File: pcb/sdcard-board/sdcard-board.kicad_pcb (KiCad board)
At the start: 2 copper layers, 82.5 x 67.3 mm, 38 parts, among them J3 SD Card Board, J4 EXPBUS1, U1 74HC123, U3 74HC00, U4 74HC00, U5 74HC163, U6 74HC00, U7 74HC165, U8 74HC595, X1 16MHz

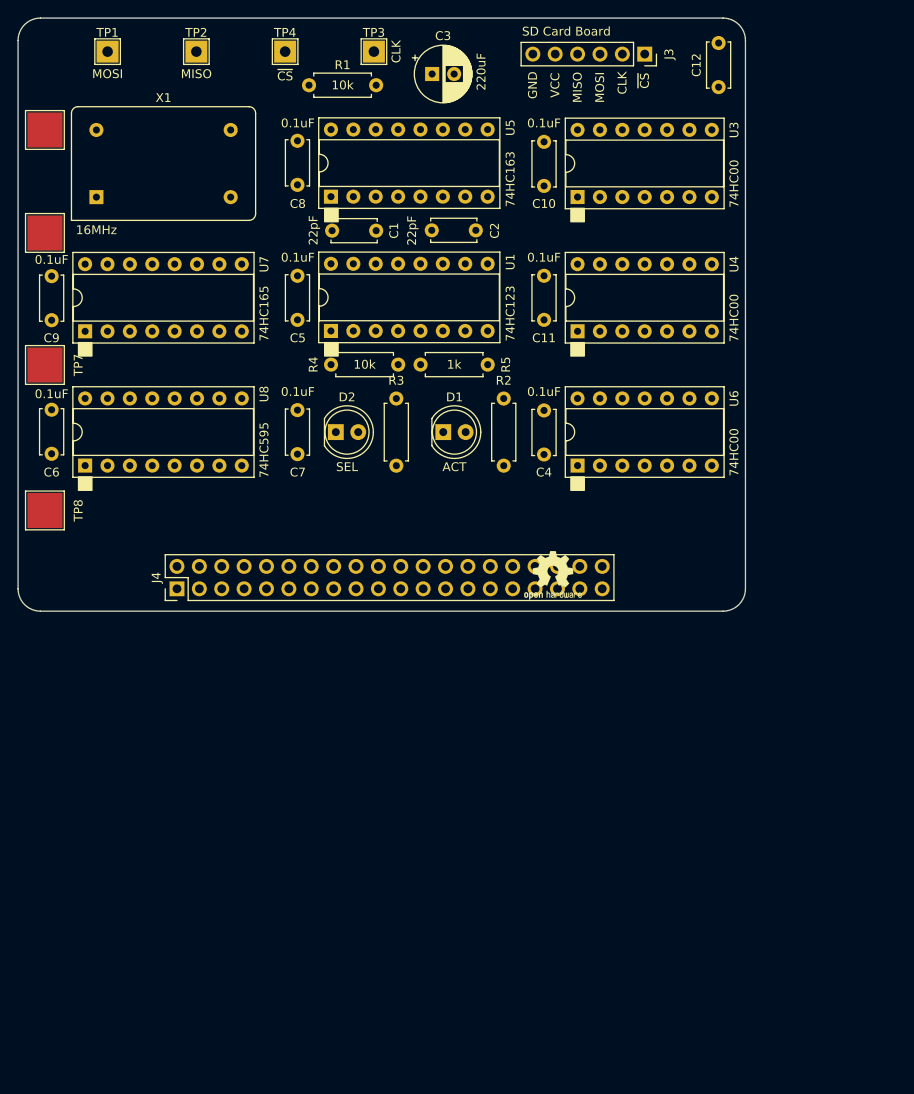
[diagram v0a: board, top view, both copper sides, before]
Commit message: Further redesigning boards
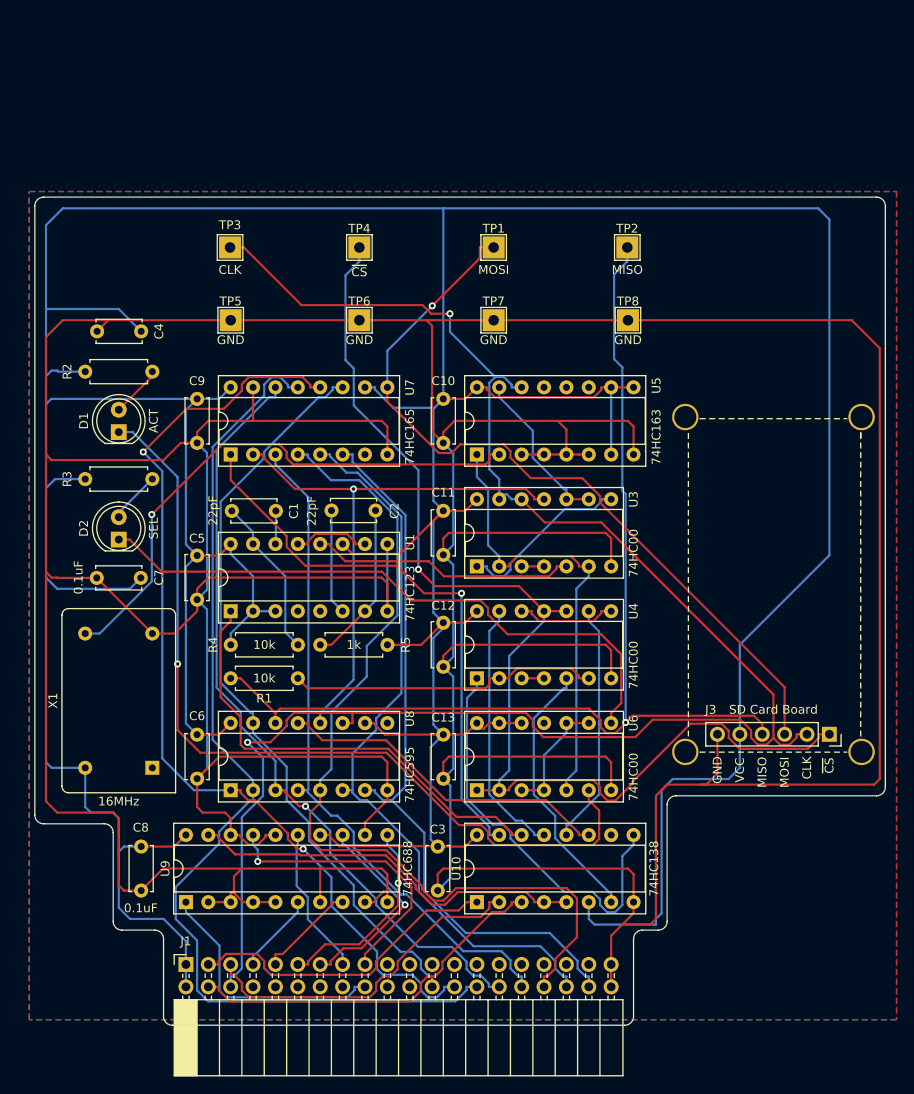
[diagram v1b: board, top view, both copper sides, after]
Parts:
- removed J4: EXPBUS1, Connector_PinHeader_2.54mm:PinHeader_2x20_P2.54mm_Vertical
- removed REF**: OSHW-Logo2_7.3x6mm_SilkScreen, Symbol:OSHW-Logo2_7.3x6mm_SilkScreen
- added C13: 0.1uF, Capacitor_THT:C_Disc_D5.0mm_W2.5mm_P5.00mm, F.Cu at (74.9, 115.6)
- added J1: EXPBUS2, Connector_PinSocket_2.54mm:PinSocket_2x20_P2.54mm_Horizontal, F.Cu at (45.7, 141.7)
- added U10: 74HC138, Package_DIP:DIP-16_W7.62mm_Socket, F.Cu at (78.7, 134.6)
- added U9: 74HC688, Package_DIP:DIP-20_W7.62mm_Socket, F.Cu at (45.7, 134.6)
- C3: value 220uF -> 0.1uF; footprint Capacitor_THT:CP_Radial_D6.3mm_P2.50mm -> Capacitor_THT:C_Disc_D5.0mm_W2.5mm_P5.00mm
- J3: footprint Connector_PinSocket_2.54mm:PinSocket_1x06_P2.54mm_Vertical -> sdcard-holder:sdcard-socket
- TP5, TP6, TP7, TP8: footprint TestPoint:TestPoint_Pad_4.0x4.0mm -> TestPoint:TestPoint_THTPad_2.5x2.5mm_Drill1.2mm
- moved C3 87.7 mm to (74.3, 128.3), turned to -90 degrees
- moved J3 80.0 mm to (118.7, 115.6)
- moved C8 77.2 mm to (40.6, 128.3), turned to -90 degrees
- moved TP8 69.6 mm to (95.9, 68.6)
- moved C12 68.3 mm to (74.9, 102.9), turned to -90 degrees
- moved R1 67.3 mm to (58.4, 109.2), turned to 180 degrees
- moved X1 65.1 mm to (41.9, 119.4), turned to 90 degrees
- moved TP2 53.7 mm to (95.8, 60.3)
- moved TP7 51.2 mm to (80.6, 68.6)
- moved TP1 49.1 mm to (80.6, 60.3)
- moved C4 47.8 mm to (40.6, 69.8), turned to 180 degrees
- moved U3 43.4 mm to (78.7, 96.5)
- moved R2 41.3 mm to (41.9, 74.4), turned to 180 degrees
- moved U4 41.0 mm to (78.7, 109.2)
- moved U8 40.4 mm to (50.8, 121.9)
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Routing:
- net GND: track 0.00 -> 735.7 mm
- net VCC: track 0.00 -> 604.3 mm
- net CLK: track 0.00 -> 204.3 mm, vias 0 -> 2
- net ~{CS}: track 0.00 -> 130.1 mm, vias 0 -> 1
- net MISO: track 0.00 -> 122.4 mm, vias 0 -> 1
- net D2: track 0.00 -> 115.9 mm
- net D1: track 0.00 -> 109.6 mm, vias 0 -> 2
- net D5: track 0.00 -> 101.2 mm
- net Net-(D1-K): track 0.00 -> 97.5 mm, vias 0 -> 1
- net D3: track 0.00 -> 89.0 mm, vias 0 -> 1
- net MOSI: track 0.00 -> 89.0 mm, vias 0 -> 1
- net D0: track 0.00 -> 85.9 mm
- net D6: track 0.00 -> 84.2 mm
- net D7: track 0.00 -> 83.4 mm
- net D4: track 0.00 -> 76.7 mm
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- added copper zone on F.Cu, net GND
- added copper zone on B.Cu, net VCC
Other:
- board size 82.5 x 67.3 mm -> 96.5 x 94 mm
